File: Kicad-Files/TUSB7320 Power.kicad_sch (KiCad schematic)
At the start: 46 parts, among them U3 TPS74401

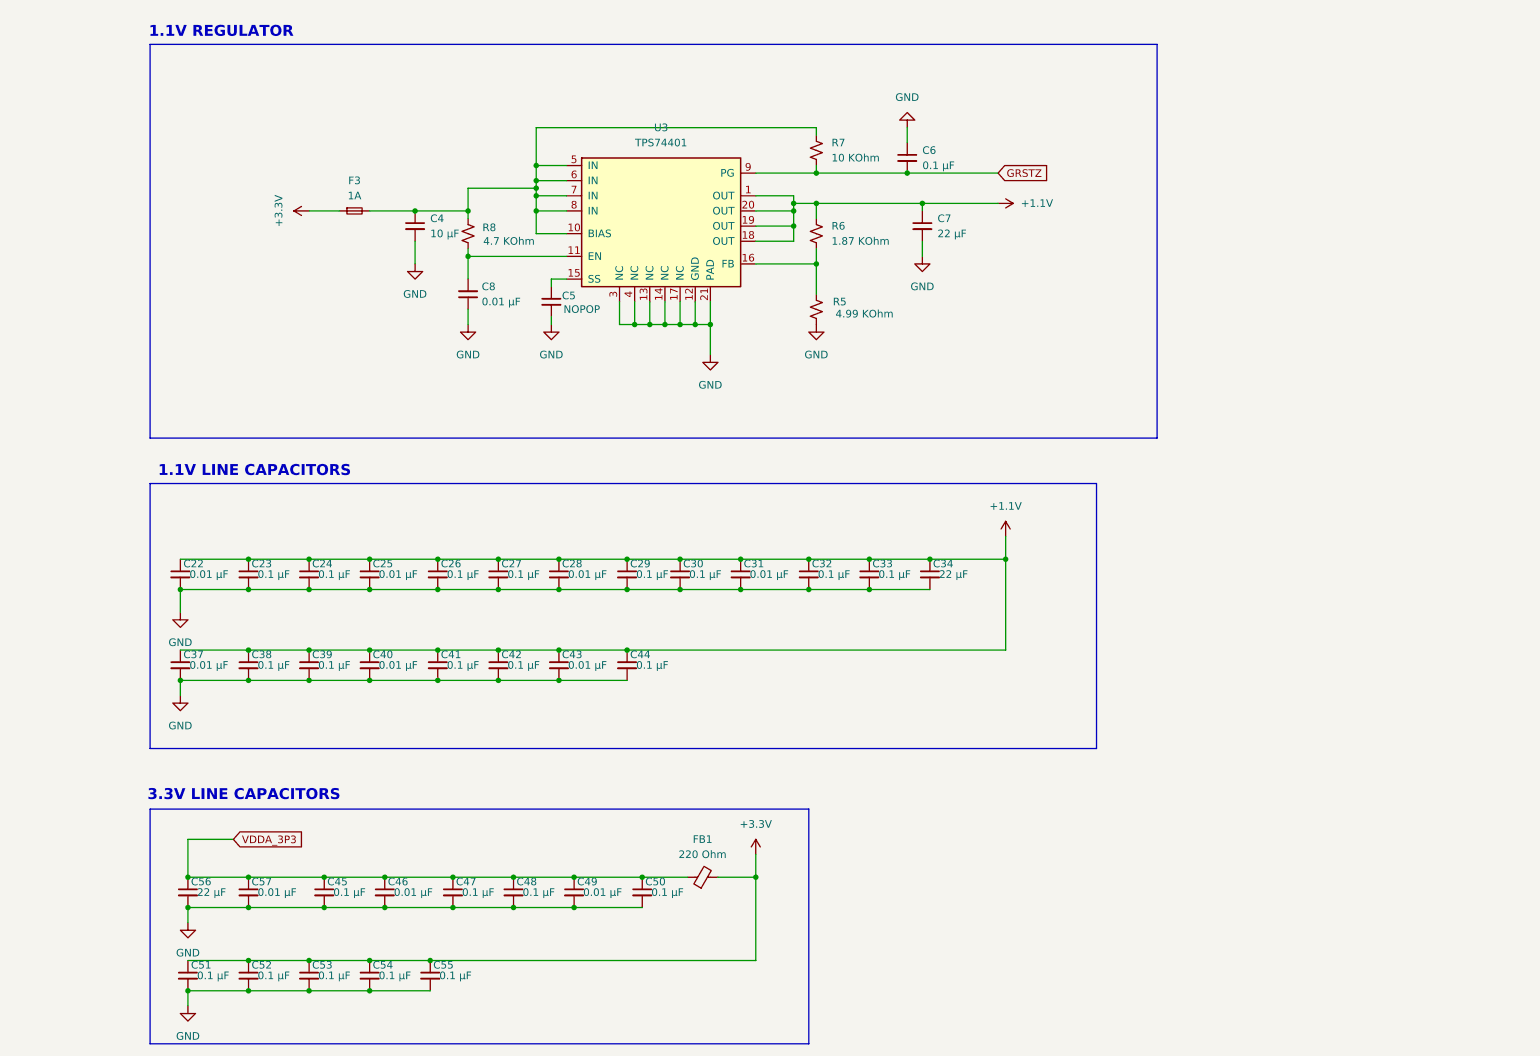
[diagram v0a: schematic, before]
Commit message: Redesigned schematic and board REV 2.0
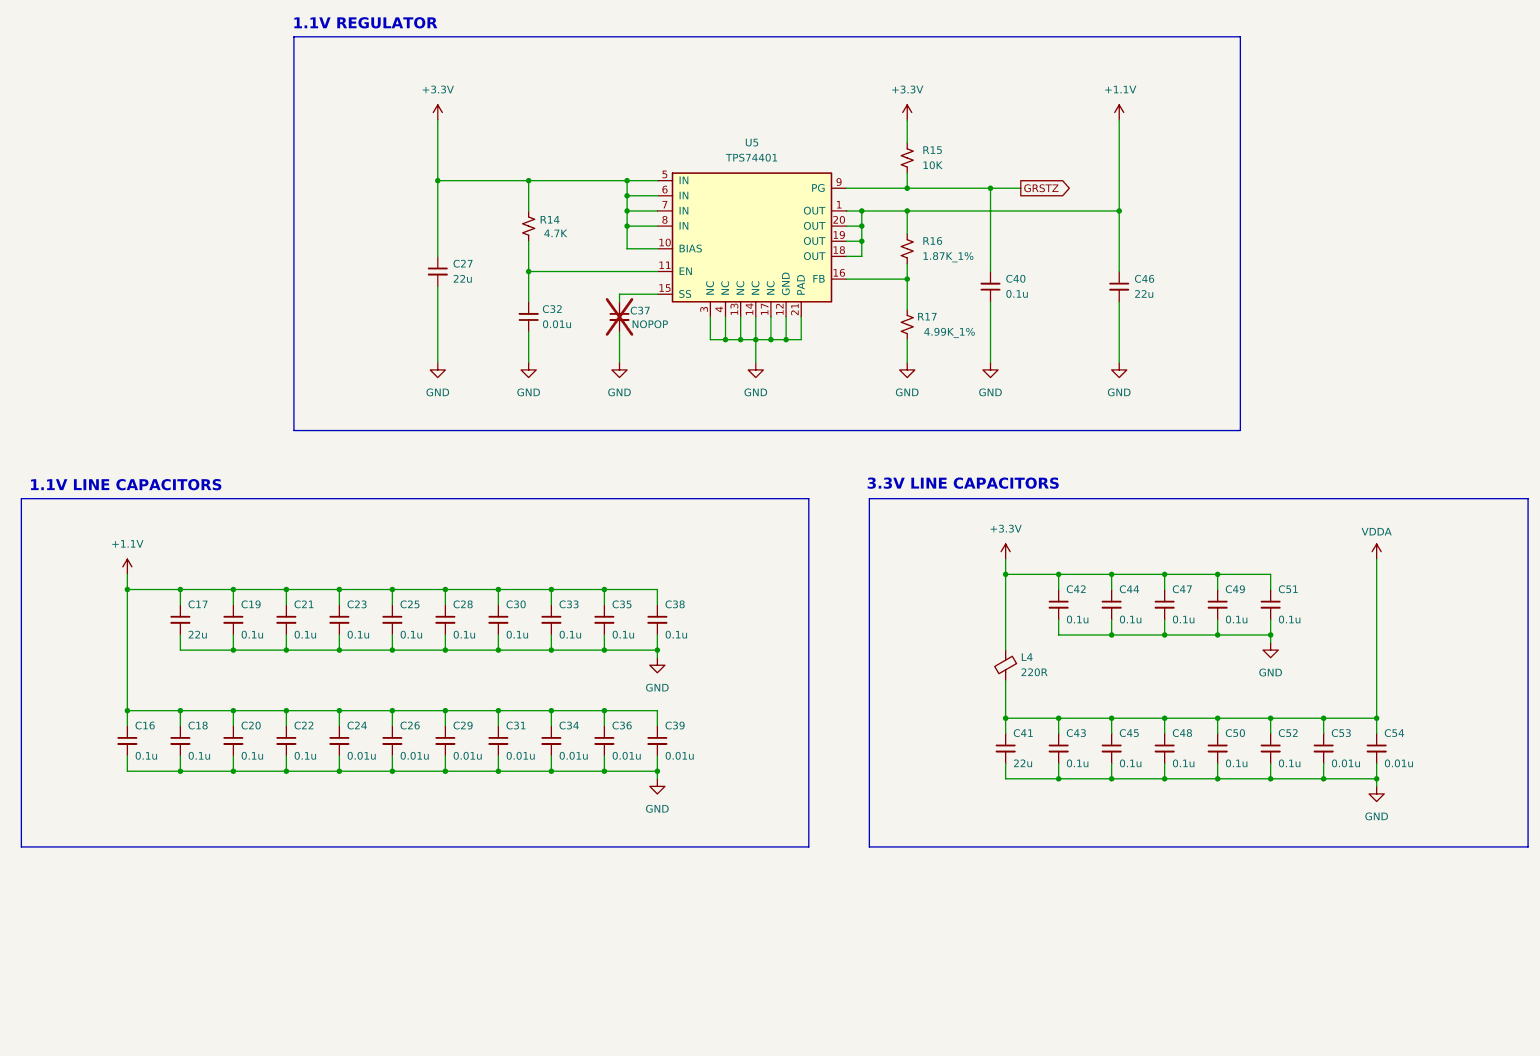
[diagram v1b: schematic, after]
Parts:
- removed C27, C32, C55: 0.1 μF, Capacitor_SMD:C_0402_1005Metric, symbol Device:C_Small
- removed C37, C40, C46, C57: 0.01 μF, Capacitor_SMD:C_0402_1005Metric, symbol Device:C_Small
- removed C56: 22 μF, Capacitor_SMD:C_0805_2012Metric, symbol Device:C_Small
- removed F3: 1A, Fuse:Fuse_0603_1608Metric, symbol Device:Fuse_Small
- removed FB1: 220 Ohm, Inductor_SMD:L_0603_1608Metric, symbol Device:FerriteBead_Small
- added C16, C18, C20, C21, C23, C35: 0.1u, Capacitor_SMD:C_0402_1005Metric, symbol Device:C_Small
- added C17: 22u, Capacitor_SMD:C_0805_2012Metric, symbol Device:C_Small
- added C36: 0.01u, Capacitor_SMD:C_0402_1005Metric, symbol Device:C_Small
- added L4: 220R, Inductor_SMD:L_0603_1608Metric, symbol Device:FerriteBead_Small
- C19: renamed from C23; value 0.1 μF -> 0.1u
- C22, C25, C28, C43, C49: value 0.01 μF -> 0.1u
- C24, C26, C29, C39, C53, C54: value 0.1 μF -> 0.01u
- C27: renamed from C4; value 10 μF -> 22u
- C30, C33, C38, C42, C44, C45, C47, C48, C50, C51, C52: value 0.1 μF -> 0.1u
- C31: value 0.01 μF -> 0.01u
- C32: renamed from C8; value 0.01 μF -> 0.01u
- C34: value 22 μF -> 0.01u; footprint Capacitor_SMD:C_0805_2012Metric -> Capacitor_SMD:C_0402_1005Metric
- C37: renamed from C5; footprint Capacitor_SMD:C_0402_1005Metric_Pad0.74x0.62mm_HandSolder -> Capacitor_SMD:C_0402_1005Metric; now not fitted; now left out of the parts list
- C40: renamed from C6; value 0.1 μF -> 0.1u
- C41: value 0.1 μF -> 22u; footprint Capacitor_SMD:C_0402_1005Metric -> Capacitor_SMD:C_0805_2012Metric
- C46: renamed from C7; value 22 μF -> 22u
- R14: renamed from R8; value 4.7 KOhm -> 4.7K
- R15: renamed from R7; value 10 KOhm -> 10K
- R16: renamed from R6; value 1.87 KOhm -> 1.87K_1%
- R17: renamed from R5; value 4.99 KOhm -> 4.99K_1%
- renumbered U3 to U5
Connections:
- net +1.1V: now also C16.1, C17.1, C18.1, C20.1, C21.1, C23.1, C35.1, C36.1; no longer C41.1, C42.1, C43.1, C44.1
- net +3.3V: now also C27.1, C42.1, C44.1, C47.1, C49.1, R14.1, R15.1, U5.10 (BIAS), U5.5 (IN), U5.6 (IN), U5.7 (IN), U5.8 (IN), L4.1; no longer C52.1, C53.1, C54.1
- net GND: now also C16.2, C17.2, C18.2, C20.2, C21.2, C23.2, C35.2, C36.2
- net VDDA_3P3 renamed VDDA
- net VDDA: now also C41.1, C43.1, C52.1, C53.1, C54.1, L4.2; no longer C47.1, C49.1
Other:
- company: 3mdeb Sp. z o.o    Jakub Sobota -> 3mdeb Sp. z o.o    Dominik Baroński
- title: PCI2USB -> PCI2USB TUSB7320 Power
- moved on the sheet: C19, C27, C32, C40, C46, R14, R15, R16, R17, U5
